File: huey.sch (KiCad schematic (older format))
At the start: 23 parts, among them CON1 PJ-036AH-SMT-TR, P1 TO_LEDS, P2 NPTC161KFXC-RC, P3 NPTC121KFXC-RC, P4 CONN_01X06, P5 CONN_01X02, P6 CONN_01X02, P7 CONN_01X02, Q1 MF-DSC-SOT233-BSS138, U1 FEATHER_M0_WIFI

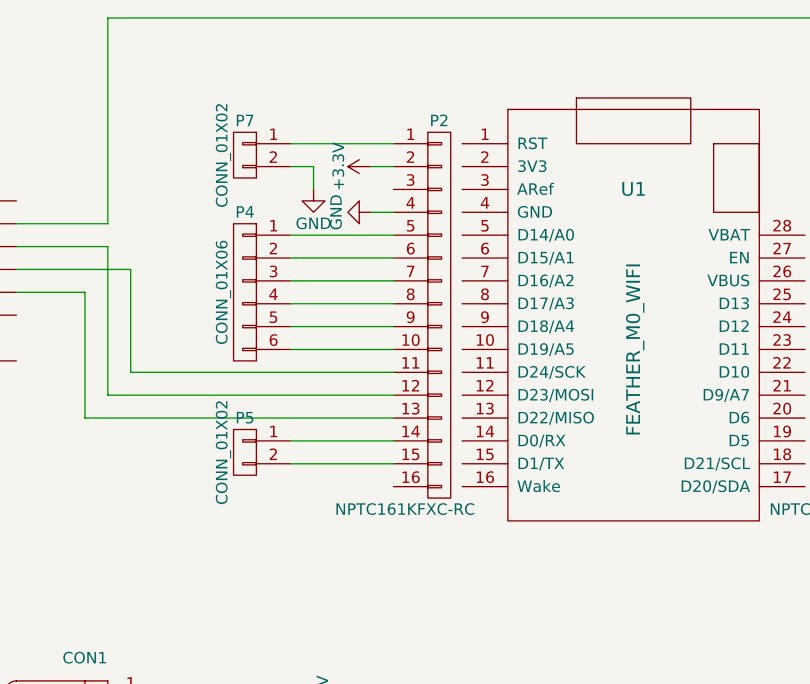
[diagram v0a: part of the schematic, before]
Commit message: Pushing final changes for rev 1.0
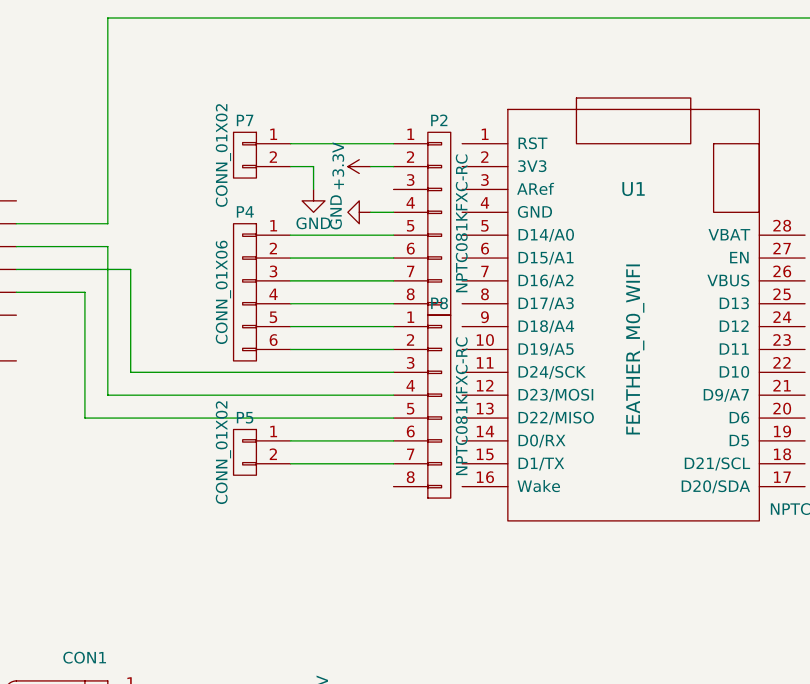
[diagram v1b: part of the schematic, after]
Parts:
- removed P2: NPTC161KFXC-RC, Huey:FEMALE_HEADER_16x1_SMD, symbol CONN_01X16
- added P2, P8: NPTC081KFXC-RC, Huey:FEMALE_HEADER_8x1_SMD, symbol CONN_01X08
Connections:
- net +3V3: now also P2.2 (P2)
- net GND: now also P2.4 (P4)
- net at SD1.3 (DI): now also P8.4 (P4)
- net at SD1.5 (SCLK): now also P8.3 (P3)
- net at SD1.7 (D0): now also P8.5 (P5)
- net at P7.1 (P1): now also P2.1 (P1)
- net at P4.6 (P6): now also P8.2 (P2)
- net at P5.1 (P1): now also P8.6 (P6)
- net at P5.2 (P2): now also P8.7 (P7)
- net at P4.1 (P1): now also P2.5 (P5)
- net at P4.2 (P2): now also P2.6 (P6)
- net at P4.3 (P3): now also P2.7 (P7)
- net at P4.4 (P4): now also P2.8 (P8)
- net at P4.5 (P5): now also P8.1 (P1)
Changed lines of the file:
@@
 	1100 4400 1000 4400
 Connection ~ 1000 4400
-$Comp
-L CONN_01X16 P2
-U 1 1 5ACB3909
-P 4250 2300
-F 0 "P2" H 4250 3150 50  0000 C CNN
-F 1 "NPTC161KFXC-RC" H 4100 1450 50  0000 C CNN
-F 2 "Huey:FEMALE_HEADER_16x1_SMD" H 4250 2300 50  0001 C CNN
-F 3 "" H 4250 2300 50  0000 C CNN
-F 4 "S5608-ND" H 4250 2300 60  0001 C CNN "Digikey"
-	1    4250 2300
-	1    0    0    -1
-$EndComp
 Wire Wire Line
 	3950 1650 4050 1650
@@
 Wire Wire Line
 	4050 1550 3600 1550
+$Comp
+L CONN_01X08 P2
+U 1 1 5ACD46B8
+P 4250 1900
+F 0 "P2" H 4250 2350 50  0000 C CNN
+F 1 "NPTC081KFXC-RC" V 4350 1900 50  0000 C CNN
+F 2 "Huey:FEMALE_HEADER_8x1_SMD" H 4250 1900 50  0001 C CNN
+F 3 "" H 4250 1900 50  0000 C CNN
+	1    4250 1900
+	1    0    0    -1
+$EndComp
+$Comp
+L CONN_01X08 P8
+U 1 1 5ACD4916
+P 4250 2700
+F 0 "P8" H 4250 3150 50  0000 C CNN
+F 1 "NPTC081KFXC-RC" V 4350 2700 50  0000 C CNN
+F 2 "Huey:FEMALE_HEADER_8x1_SMD" H 4250 2700 50  0001 C CNN
+F 3 "" H 4250 2700 50  0000 C CNN
+	1    4250 2700
+	1    0    0    -1
+$EndComp
 $EndSCHEMATC
